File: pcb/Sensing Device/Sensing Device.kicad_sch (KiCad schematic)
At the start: 19 parts, among them J1 PWR_PAD, J2 ID_PAD, SW1 SW_SPST, SW2 SW_SPDT, U2 TLV493D

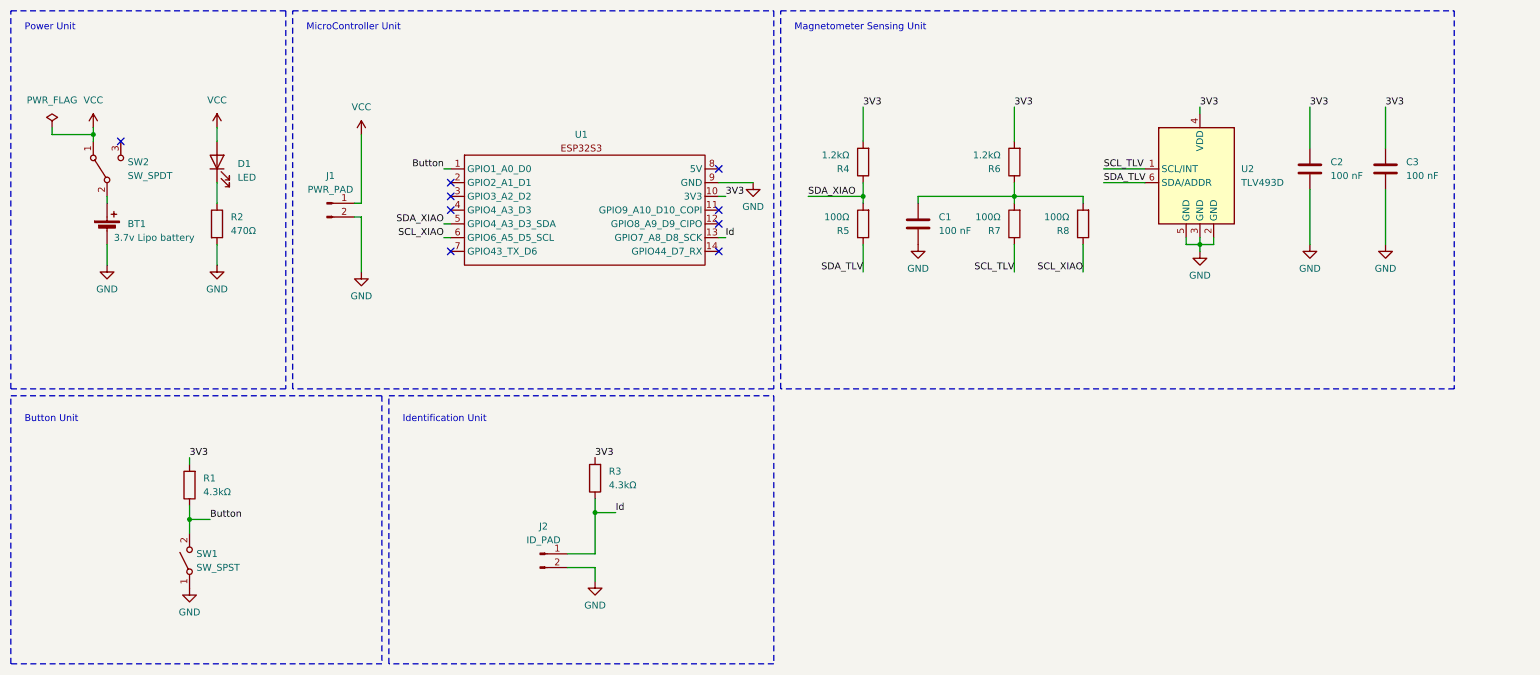
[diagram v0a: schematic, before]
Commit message: power management
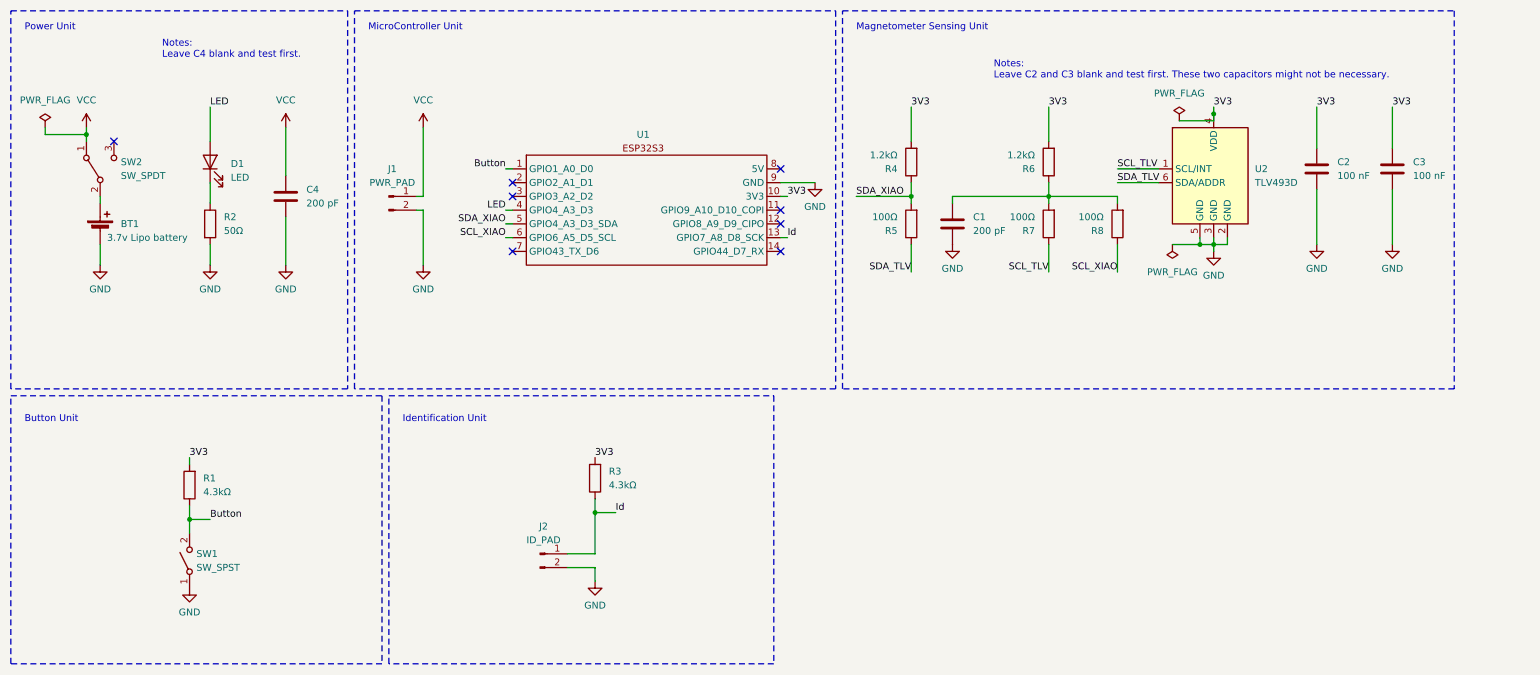
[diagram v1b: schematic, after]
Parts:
- added C4: 200 pF, Capacitor_SMD:C_0805_2012Metric_Pad1.18x1.45mm_HandSolder, symbol Device:C
- C1: value 100 nF -> 200 pF
- R2: value 470Ω -> 50Ω
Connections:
- net GND: now also C4.2
- net VCC: now also C4.1; no longer D1.2 (A)
- net LED: now reaches U1.4 (GPIO4_A3_D3)
- net LED: now also D1.2 (A)
- no-connect marks 9 -> 8
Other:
- note added: "Notes: Leave C2 and C3 blank and test first. These two capacitors might not be necessary."
- note added: "Notes: Leave C4 blank and test first."
- moved on the sheet: BT1, C1, C2, C3, D1, J1, R2, R4, R5, R6, R7, R8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
